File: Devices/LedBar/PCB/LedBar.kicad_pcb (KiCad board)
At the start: 2 copper layers, 63.5 x 99.3 mm, 167 parts, among them J1001 Conn_02x06_Odd_Even, J1002 Conn_02x06_Odd_Even, J1101 strip1_RGBW, J1102 Conn_01x05, J1103 Strip1_BRG, J1201 strip2_RGBW, J1202 Conn_02x06_Odd_Even, J1203 Strip3_RGBW, J1204 Strip2_BRG, J1205 Strip3_BRG, J1301 Conn_01x05, J1302 Strip4_RGBW, J1303 Strip4_BRG, J301 12VDC/5A, J401 RS485, J501 Left, J502 Center, J503 Right, J601 0-10V(1), J701 AVR-ISP-6, Q501 Si2302DS, Q502 Si2302DS, Q503 Si2302DS, Q504 Si2302DS, Q505 Si2302DS, Q506 Si2302DS, Q507 Si2302DS, Q508 Si2302DS, Q509 Si2302DS, Q510 Si2302DS, Q511 Si2302DS, Q512 Si2302DS, Q513 Si2302DS, Q514 Si2302DS, Q515 Si2302DS, Q516 Si2302DS, SW701 button, SW702 reset, SW703 SW_DIP_x05, U301 INA219AxD, U302 AMS1117-5.0, U401 ISO3082DW, U402 B0505S-1W-SIP4, U501 PCA9685PW, U601 LM393, U701 ATmega328P-AU, U901 DS1307Z+, Y701 14.7456Mhz, Y901 23.768kHz

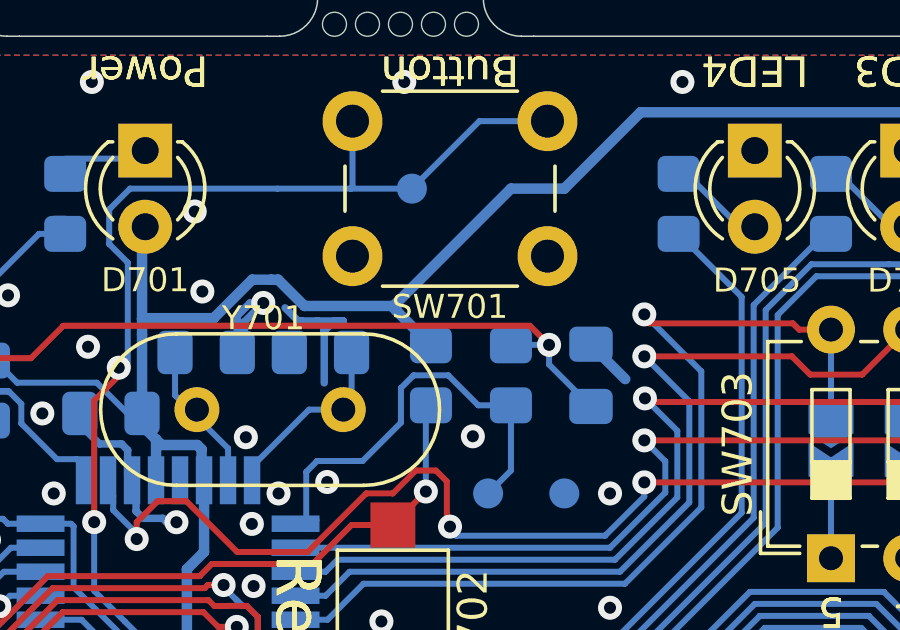
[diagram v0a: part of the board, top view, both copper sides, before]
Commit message: Working on LEDs and Button for the Case
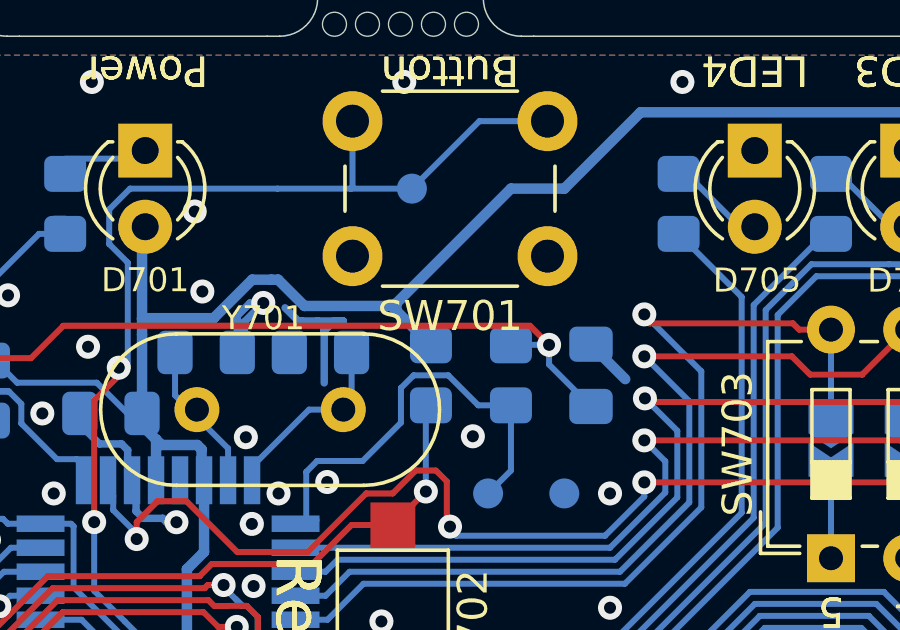
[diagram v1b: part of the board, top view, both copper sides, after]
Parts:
- SW701: footprint Button_Switch_THT:SW_PUSH_6mm_H4.3mm -> Button_Switch_THT:SW_PUSH_6mm_H8mm
